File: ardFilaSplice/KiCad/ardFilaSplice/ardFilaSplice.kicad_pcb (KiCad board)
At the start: 2 copper layers, 88.3 x 54.6 mm, 19 parts, among them J1 2-pin_fan_output_header, J2 3-pin_KY-019_relay_header, K1 SANYOU_SRD_Form_C, Q1 20N6003, U1 KY-040_Rotary_Encoder, U2 2-pole_power_in_screw_terminal, U3 Arduino_Mini_Pro, U4 TM1637_4x7-segment_display, U5 L7805, U6 4-pole_Heater_thermistor_scre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

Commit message: kicad6, moved espscale
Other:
- net class Default removed
- net class Power removed

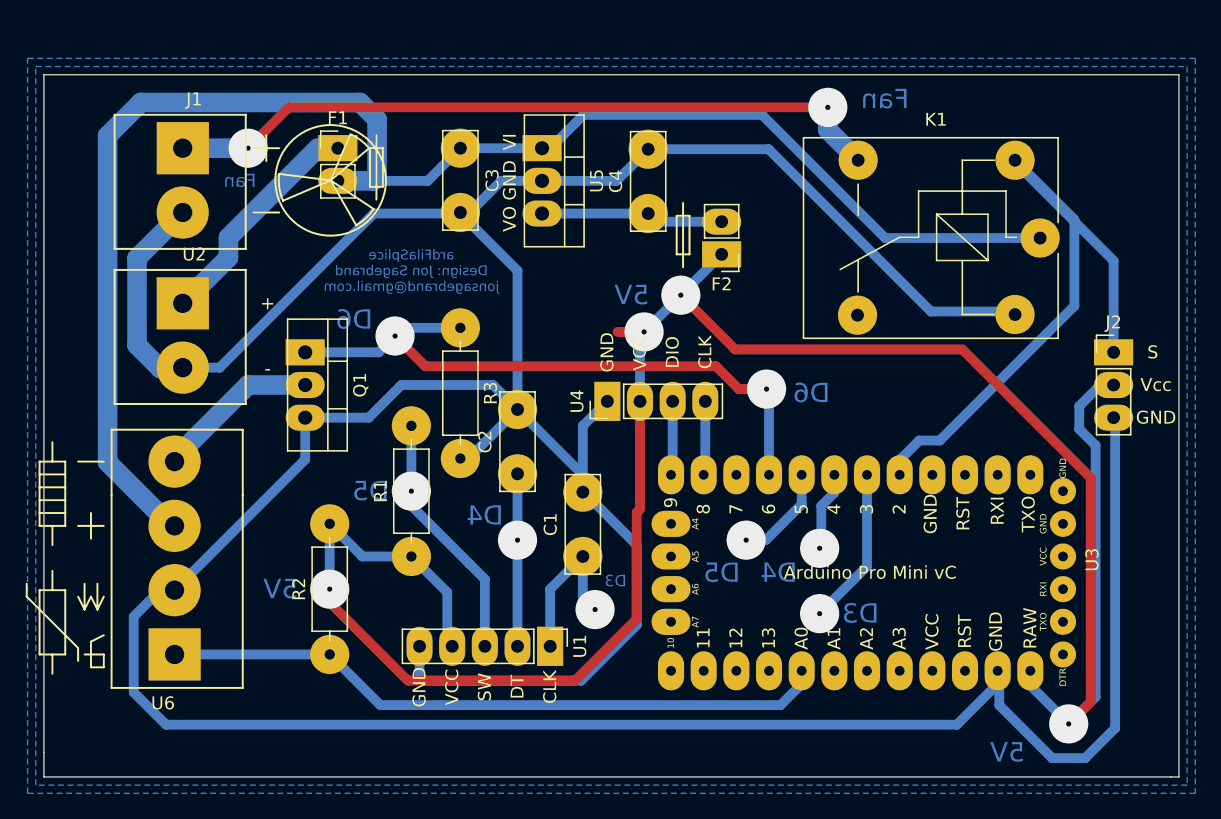
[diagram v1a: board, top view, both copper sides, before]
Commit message: new pcb
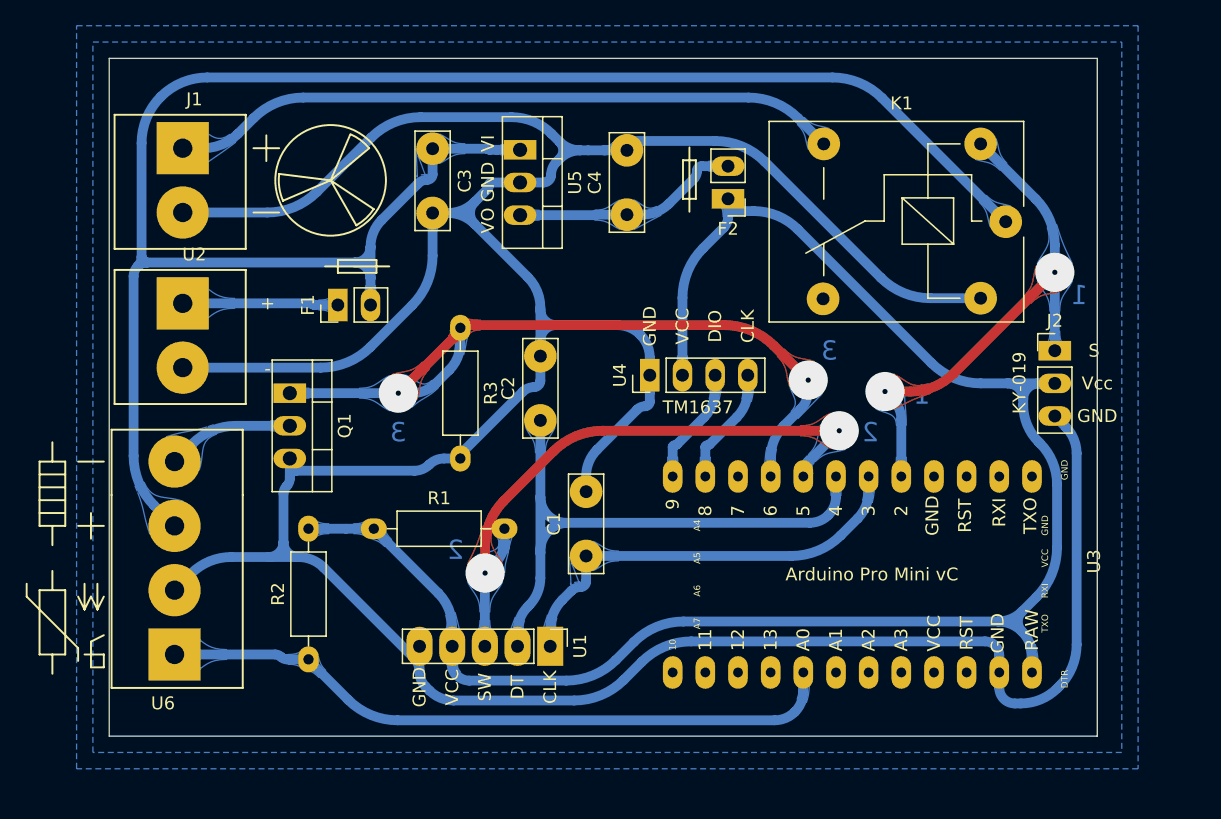
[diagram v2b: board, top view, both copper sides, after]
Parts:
- R1, R2, R3: footprint My_Misc:R_Axial_DIN0207_L6.3mm_D2.5mm_P10.16mm_Horizontal_larger_pads -> My_Misc:R_Axial_DIN0207_L6.3mm_D2.5mm_P10.16mm_Horizontal_large
- U3: footprint My_Arduino:Arduino_Pro_Mini_vC_larger_pads -> My_Arduino:Arduino_Pro_Mini_vC_only_sides_larger_pads
- moved F1 12.2 mm to (97.8, 63.6), turned to 90 degrees
- moved J2 4.57 mm to (153.5, 67.2)
- moved C2 4.52 mm to (113.5, 72.6)
- moved F2 4.35 mm to (128.1, 55.4)
- moved U3 4.06 mm to (151.8, 77.0)
- moved U4 3.88 mm to (122.0, 69.1)
- moved R1 3.63 mm to (100.6, 81.0), turned to 0 degrees
- moved Q1 3.39 mm to (94.1, 70.5)
- moved K1 2.96 mm to (149.7, 57.1)
- moved C3 2.16 mm to (105.2, 51.5)
- moved U5 1.71 mm to (112.0, 51.6)
- moved R2 1.69 mm to (95.5, 91.2)
- moved C4 1.65 mm to (120.3, 56.6)
- moved C1 0.26 mm to (117.1, 83.1)
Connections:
- K1 pad 4: Net-(K1-Pad4) -> unconnected-(K1-Pad4)
- U3 pad 1: Net-(U3-Pad1) -> unconnected-(U3-Pad1)
- U3 pad 10: Net-(U3-Pad10) -> unconnected-(U3-Pad10)
- U3 pad 15: Net-(U3-Pad15) -> unconnected-(U3-Pad15)
- U3 pad 16: Net-(U3-Pad16) -> unconnected-(U3-Pad16)
- U3 pad 17: Net-(U3-Pad17) -> unconnected-(U3-Pad17)
- U3 pad 18: Net-(U3-Pad18) -> unconnected-(U3-Pad18)
- U3 pad 19: Net-(U3-Pad19) -> unconnected-(U3-Pad19)
- U3 pad 2: Net-(U3-Pad2) -> unconnected-(U3-Pad2)
- U3 pad 21: Net-(U3-Pad21) -> unconnected-(U3-Pad21)
- U3 pad 22: Net-(U3-Pad22) -> unconnected-(U3-Pad22)
- U3 pad 23: Net-(U3-Pad23) -> unconnected-(U3-Pad23)
- U3 pad 24: Net-(U3-Pad24) -> unconnected-(U3-Pad24)
- U3 pad 3: Net-(U3-Pad3) -> unconnected-(U3-Pad3)
- U3 pad 4: Net-(U3-Pad4) -> unconnected-(U3-Pad4)
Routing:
- net +5V: track 175.6 -> 139.8 mm, vias 4 -> 0
- net Net-(C2-Pad1): track 19.5 -> 48.1 mm, vias 2 -> 0
- net GND: track 320.6 -> 295.9 mm
- net +12Vf: track 123.5 -> 147.9 mm
- net Net-(R1-Pad2): track 27.3 -> 48.4 mm
- net Net-(Q1-Pad1): track 50.7 -> 60.5 mm
- net Net-(J2-Pad1): track 51.3 -> 42.1 mm, vias 0 -> 2
- net Net-(C1-Pad1): track 25.3 -> 33.8 mm, vias 2 -> 0
- net +12V: track 18.0 -> 12.1 mm
- net Net-(J1-Pad1): track 56.6 -> 52.3 mm, vias 2 -> 0
- net Net-(C4-Pad1): track 14.2 -> 17.8 mm
- net Net-(U3-Pad11): track 5.71 -> 9.18 mm
- net Net-(U3-Pad12): track 5.71 -> 9.18 mm
- net +12Vh: track 12.5 -> 9.88 mm
- net Net-(R2-Pad1): track 52.2 -> 53.5 mm
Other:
- board size 88.3 x 54.6 mm -> 76.8 x 52.7 mm
- board text added: "1"
- board text added: "2"
- board text added: "3"
- board text removed: "5V"
- board text removed: "D3"
- board text removed: "D4"
- board text removed: "D5"
- board text removed: "D6"
- board text removed: "Fan"
- board text removed: "ardFilaSplice Design: Jon Sagebrand jonsagebrand@gmail.com"
